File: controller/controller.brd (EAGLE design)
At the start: 84 x 44 mm, 47 parts, among them IC1 MEGA8-P, IC2 FT230XS, IC3 LM50, T1 2N3904, X1 MINI-USB_SHIELD5P2-32005-601, Y1 32.768kHz

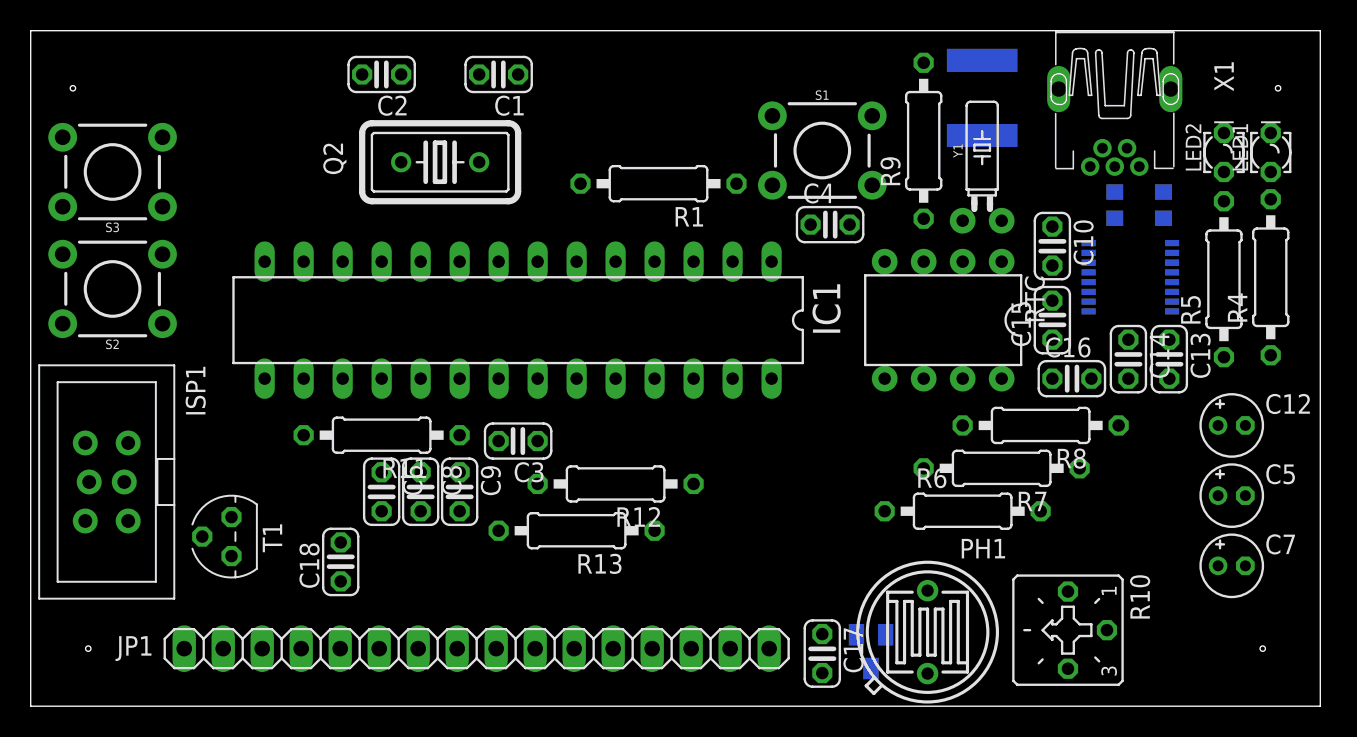
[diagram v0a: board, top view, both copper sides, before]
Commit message: Update
Completed the controller design
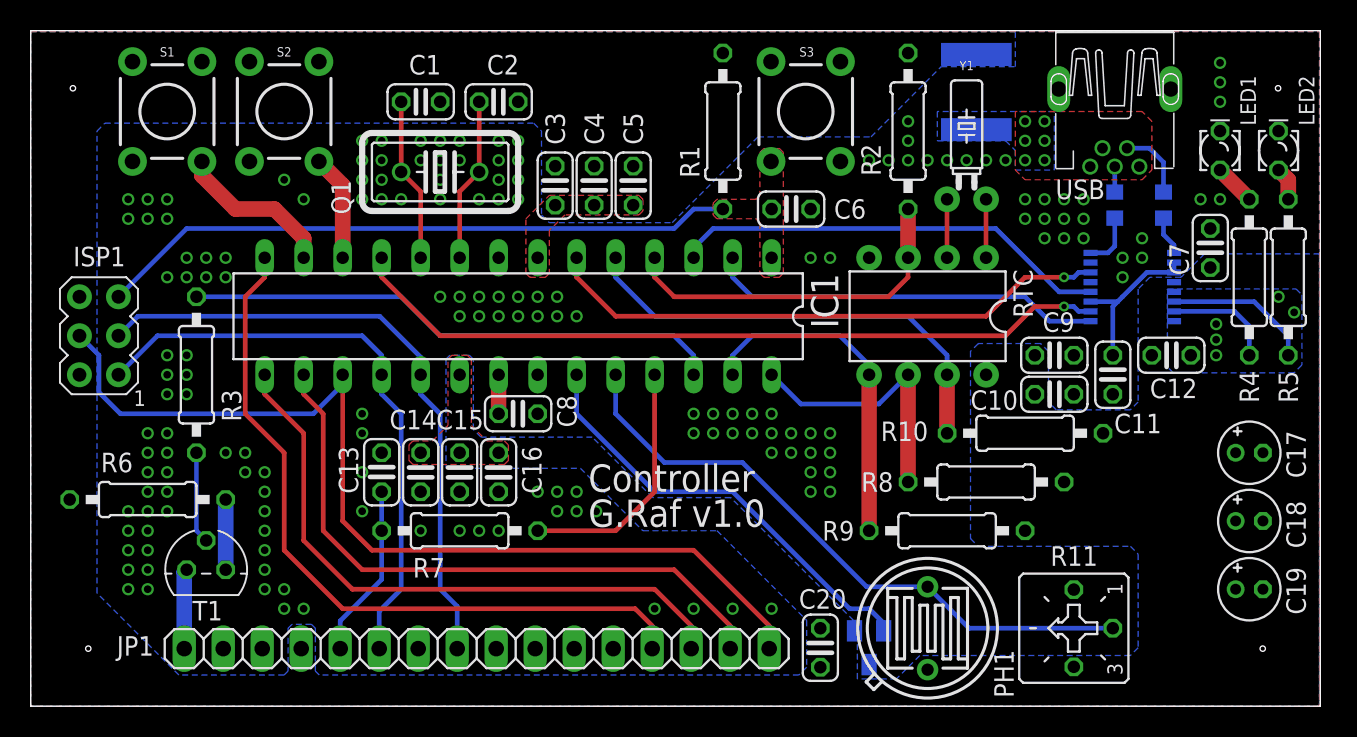
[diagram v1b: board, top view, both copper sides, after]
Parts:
- removed IC2: FT230XS, ftdichip:SSOP16
- removed IC3: LM50, linear:SOT23
- removed Q2: (no value), crystal:HC18U-V
- removed R12: 3k3, rcl:0207/10
- removed R13: 10k, rcl:0207/10
- added C11, C20: 100n, rcl:C025-024X044
- added C19: 47u, rcl:E1,8-4
- added IC100: LM50, linear:SOT23
- added IC101: FT230XS, ftdichip:SSOP16
- added Q1: (no value), crystal:HC18U-V
- added R100, R101: 27, rcl:R0603
- C12: value 4u7 -> 10n; device rcl:E1,8-4 -> rcl:C025-024X044
- C13: value 100n -> 470n
- C14, C15: value 10n -> 100n
- C16, C4: value 100n -> 10n
- C17: value 100n -> 4u7; device rcl:C025-024X044 -> rcl:E1,8-4
- C18: value 470n -> 47u; device rcl:C025-024X044 -> rcl:E1,8-4
- C5, C7: value 47u -> 100n; device rcl:E1,8-4 -> rcl:C025-024X044
- ISP1: value AVRISP-BOX -> AVRISP-6; device adafruit:AVRISP-BOX -> adafruit:AVRISP
- R10: value 100k -> 10k; device pot:CT6 -> rcl:0207/10
- R11: value Blue/White/Green=80/Amber=180 -> 100k; device rcl:0207/10 -> pot:CT6
- R2: value 27 -> 10k; device rcl:R0603 -> rcl:0207/10
- R3: value 27 -> 3k3; device rcl:R0603 -> rcl:0207/10
- R6: value 3k3 -> Blue/White/Green=80/Amber=180
- R7: value 3k3 -> 10k
- R8, R9: value 10k -> 3k3
- moved R3 64.0 mm to (10.8, 21.6), flipped to the top, turned to 270 degrees
- moved C18 59.2 mm to (79.4, 12.1), turned to 0 degrees
- moved R6 53.1 mm to (7.62, 13.5)
- moved C13 51.8 mm to (22.9, 15.2), turned to 90 degrees
- moved R11 46.8 mm to (67.9, 5.08), turned to 90 degrees
- moved C14 46.7 mm to (25.4, 15.2)
- moved S3 45.3 mm to (50.5, 38.7), turned to 90 degrees
- moved C5 43.9 mm to (39.2, 33.9), turned to 90 degrees
- moved S1 42.7 mm to (8.89, 38.7), turned to 90 degrees
- moved C15 39.9 mm to (27.9, 15.2), turned to 270 degrees
- moved C9 39.7 mm to (66.7, 22.9), turned to 0 degrees
- moved C16 37.8 mm to (30.5, 15.2), turned to 270 degrees
- moved R7 35.5 mm to (27.9, 11.4)
- moved C6 32.4 mm to (49.5, 32.4), turned to 0 degrees
- moved C17 30.7 mm to (79.4, 16.5), turned to 0 degrees
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- renumbered X1 to USB
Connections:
- net N$12 renamed V_BUS
- net ADC0: now also IC100.2; no longer IC3.2
- net ADC1: now also R11.S; no longer R10.S
- net CONT: now also C13.1, R7.2; no longer C18.1, R13.2
- net CTS: now also IC101.6; no longer IC2.6
- net E: now also IC1.19, ISP1.3; no longer IC1.18, ISP1.1
- net GND: now also C1.2, C10.2, C11.1, C12.2, C17.-, C18.-, C19.-, C2.1, C20.2, C3.2, C5.2, C7.2, C8.1, IC100.3, IC101.13, IC101.5, R11.A, S3.3; no longer C1.1, C10.1, C12.-, C17.2, C18.2, C2.2, C3.1, C5.-, C7.-, C8.2, IC2.13, IC2.5, IC3.3, R10.A, S3.1
- net INT0: now also R2.1, RTC.3; no longer R8.2, RTC.7
- net INT1: now also R10.2, RTC.7; no longer R9.1, RTC.3
- net LIGHT: now also R3.1; no longer R12.1
- net N$1: now also C2.2, Q1.2; no longer C1.2, Q2.2
- net N$10: now also IC101.9, R100.1; no longer IC2.9, R3.1
- net N$11: now also C11.2, IC101.10, IC101.11, IC101.3; no longer C10.2, IC2.10, IC2.11, IC2.3
- net N$13: now also IC101.14; no longer IC2.14
- net N$18: now also R3.2; no longer R12.2
- net N$19: now also R6.2; no longer R11.2
- net N$2: now also C1.1, Q1.1; no longer C2.1, Q2.1
- net N$20: now also R9.2; no longer R7.2
- net N$21: now also R8.1; no longer R6.1
- net N$3: now also R100.2; no longer R3.2
- net N$4: now also C8.2; no longer C3.2
- net N$5: now also IC101.15; no longer IC2.15
- net N$6: now also R101.1; no longer R2.1
- net N$7: now also S2.3; no longer S3.3
- net N$8: now also S1.3; no longer S2.3
- net N$9: now also IC101.8, R101.2; no longer IC2.8, R2.2
- net PWM: now also R7.1; no longer R13.1
- net RESET: now also C6.1, S3.1; no longer C4.1, S1.3
- net RS: now also IC1.18, ISP1.1; no longer IC1.19, ISP1.3
- net RTS: now also IC101.2; no longer IC2.2
- net RXD: now also IC101.4; no longer IC2.4
- net TXD: now also IC101.1; no longer IC2.1
- net VCC: now also C10.1, C12.1, C17.+, C18.+, C19.+, C20.1, C3.1, C4.1, C5.1, C7.1, IC100.1, IC101.12, R10.1, R11.E, R2.2, R6.1, R8.2, R9.1; no longer C12.+, C13.1, C17.1, C5.+, C6.1, C7.+, C8.1, IC2.12, IC3.1, R10.E, R11.1, R6.2, R7.1, R8.1, R9.2
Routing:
- net DB7: track 0.00 -> 63.7 mm
- net RTS: track 0.00 -> 49.9 mm, vias 0 -> 1
- net DB4: track 0.00 -> 48.1 mm
- net RESET: track 0.00 -> 41.7 mm
- net E: track 0.00 -> 41.3 mm
- net DB6: track 0.00 -> 41.3 mm
- net DB5: track 0.00 -> 40.9 mm
- net ADC1: track 0.00 -> 40.7 mm
- net RS: track 0.00 -> 39.0 mm
- net CTS: track 0.00 -> 37.0 mm, vias 0 -> 1
- net LIGHT: track 0.00 -> 35.2 mm
- net INT1: track 0.00 -> 30.0 mm
- net RXD: track 0.00 -> 28.7 mm
- net ADC0: track 0.00 -> 28.7 mm
- net TXD: track 0.00 -> 25.8 mm
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- added copper zone on layer 1, net GND
- added copper zone on layer 16, net GND
- added copper zone on layer 1, net RESET
- added copper zone on layer 1, net VCC
- added copper zone on layer 16, net VCC
- added copper zone on layer 1, net V_BUS
- added copper zone on layer 16, net V_BUS
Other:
- board text added: "Controller"
- board text added: "G.Raf v1.0"
